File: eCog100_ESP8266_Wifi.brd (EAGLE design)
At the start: 48 x 28 mm, 1 part

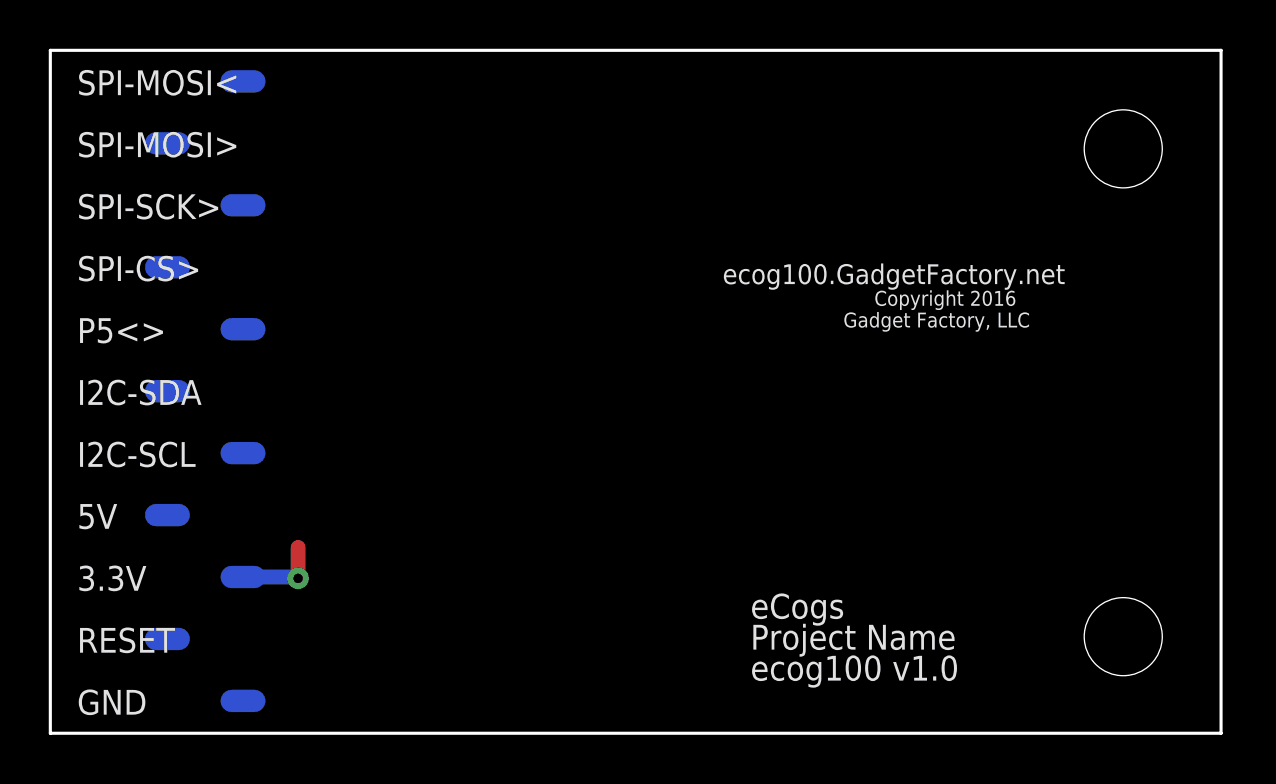
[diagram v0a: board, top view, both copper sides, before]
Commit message: V1.1
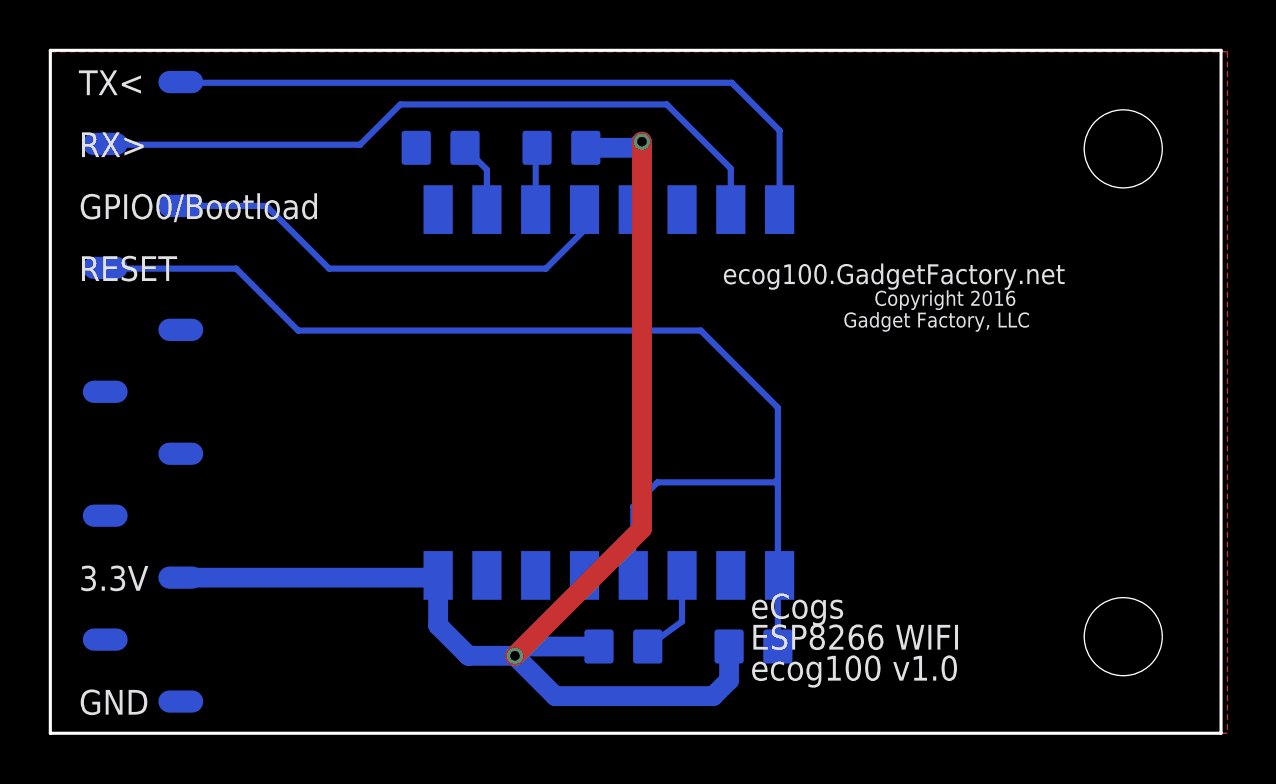
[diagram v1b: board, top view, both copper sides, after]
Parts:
- added R1, R2, R3, R4: 10K, GadgetFactory:0805
- added X1: (no value), adafruit:ESP-12
- ECOG: value ECOG_BUSES_ROWECOG_BUSES_SMD -> ECOG_GENERAL_ROWECOG_GENERAL_SMD; device eCogs:ECOG_BUSES_SMD -> eCogs:ECOG_GENERAL_SMD
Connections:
- new net GPIO0/BOOTLOAD: ECOG.3, X1.12
- new net N$3: R1.1, X1.11
- new net N$4: R2.2, X1.10
- new net N$5: R4.1, X1.3
- new net RESET: ECOG.4, R3.1, X1.1, X1.4
- new net RX: ECOG.2, X1.15
- new net TX: ECOG.1, X1.16
- net 3V3: now also R1.2, R3.2, R4.2, X1.8
- net GND: now also R2.1, X1.9
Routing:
- net 3V3: track 3.55 -> 56.7 mm, vias 1 -> 2
- net RESET: track 0.00 -> 49.1 mm
- net RX: track 0.00 -> 29.1 mm
- net TX: track 0.00 -> 28.6 mm
- net GPIO0/BOOTLOAD: track 0.00 -> 19.1 mm
- net N$5: track 0.00 -> 3.63 mm
- net N$4: track 0.00 -> 2.90 mm
- net N$3: track 0.00 -> 2.56 mm
- added copper zone on layer 1, net GND
- removed copper zone on layer 1, net 3V3
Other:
- board text added: "ESP8266 WIFI"
- board text added: "GPIO0/Bootload"
- board text added: "RX>"
- board text added: "TX<"
- board text removed: "5V"
- board text removed: "I2C-SCL"
- board text removed: "I2C-SDA"
- board text removed: "P5<>"
- board text removed: "Project Name"
- board text removed: "SPI-CS>"
- board text removed: "SPI-MOSI<"
- board text removed: "SPI-MOSI>"
- board text removed: "SPI-SCK>"

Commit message: Latest updated to V1.4
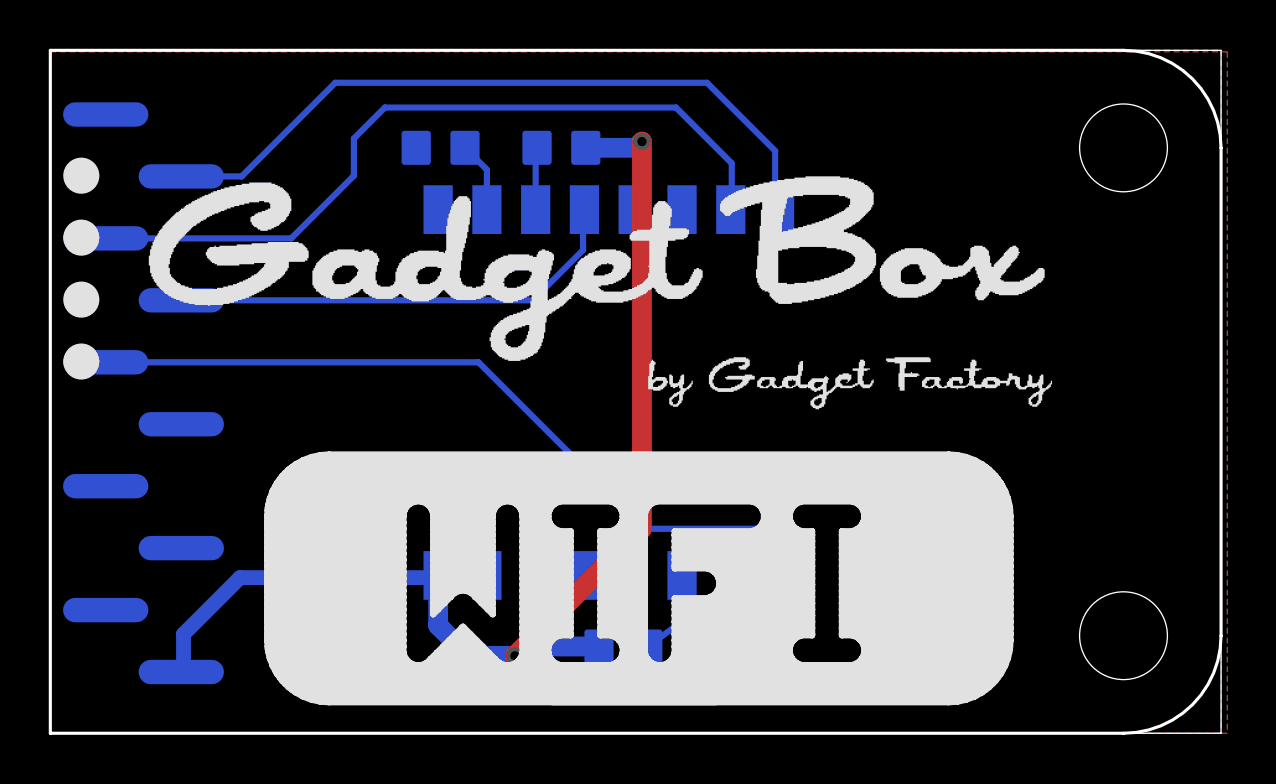
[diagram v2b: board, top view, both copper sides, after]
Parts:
- added U$1: (no value), GadgetFactory:GADGETBOX_TEXT
- added U$2, U$3, U$4, U$5: (no value), eCogs:LEGEND_DIO
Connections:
- net GPIO0/BOOTLOAD: now also ECOG.G2; no longer ECOG.3
- net RESET: now also ECOG.G3; no longer ECOG.4
- net RX: now also ECOG.G1; no longer ECOG.2
- net TX: now also ECOG.G0; no longer ECOG.1
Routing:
- net RESET: track 49.1 -> 37.3 mm
- net RX: track 29.1 -> 31.6 mm
- net 3V3: track 56.7 -> 59.1 mm
- net TX: track 28.6 -> 29.6 mm
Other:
- board text added: "GPIO0 Bootload"
- board text added: "ecog100 v1.1"
- board text removed: "GPIO0/Bootload"
- board text removed: "ecog100 v1.0"
